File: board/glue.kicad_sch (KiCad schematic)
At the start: 25 parts, among them J1 Conn_01x05_Pin, J8 SD_Card_Receptacle, U12 GLUE, U13 SN74LVC245APW, U14 LD1117V33

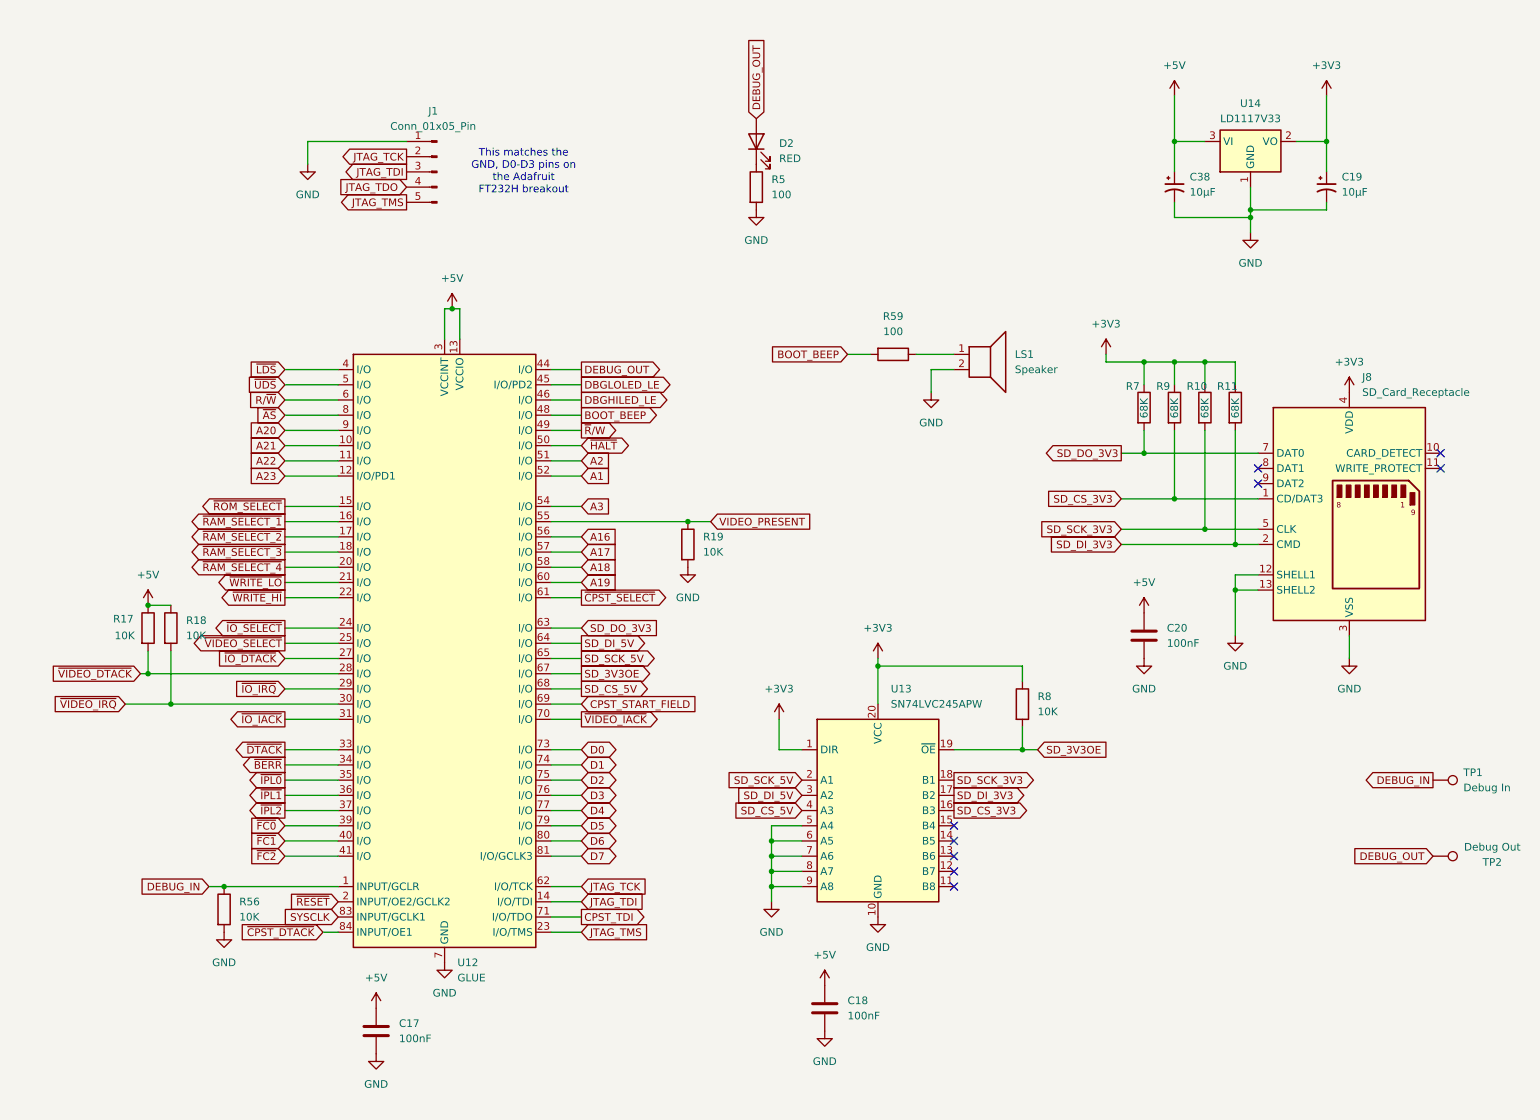
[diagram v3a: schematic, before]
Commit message: checkpoint before reordering 1508 inputs
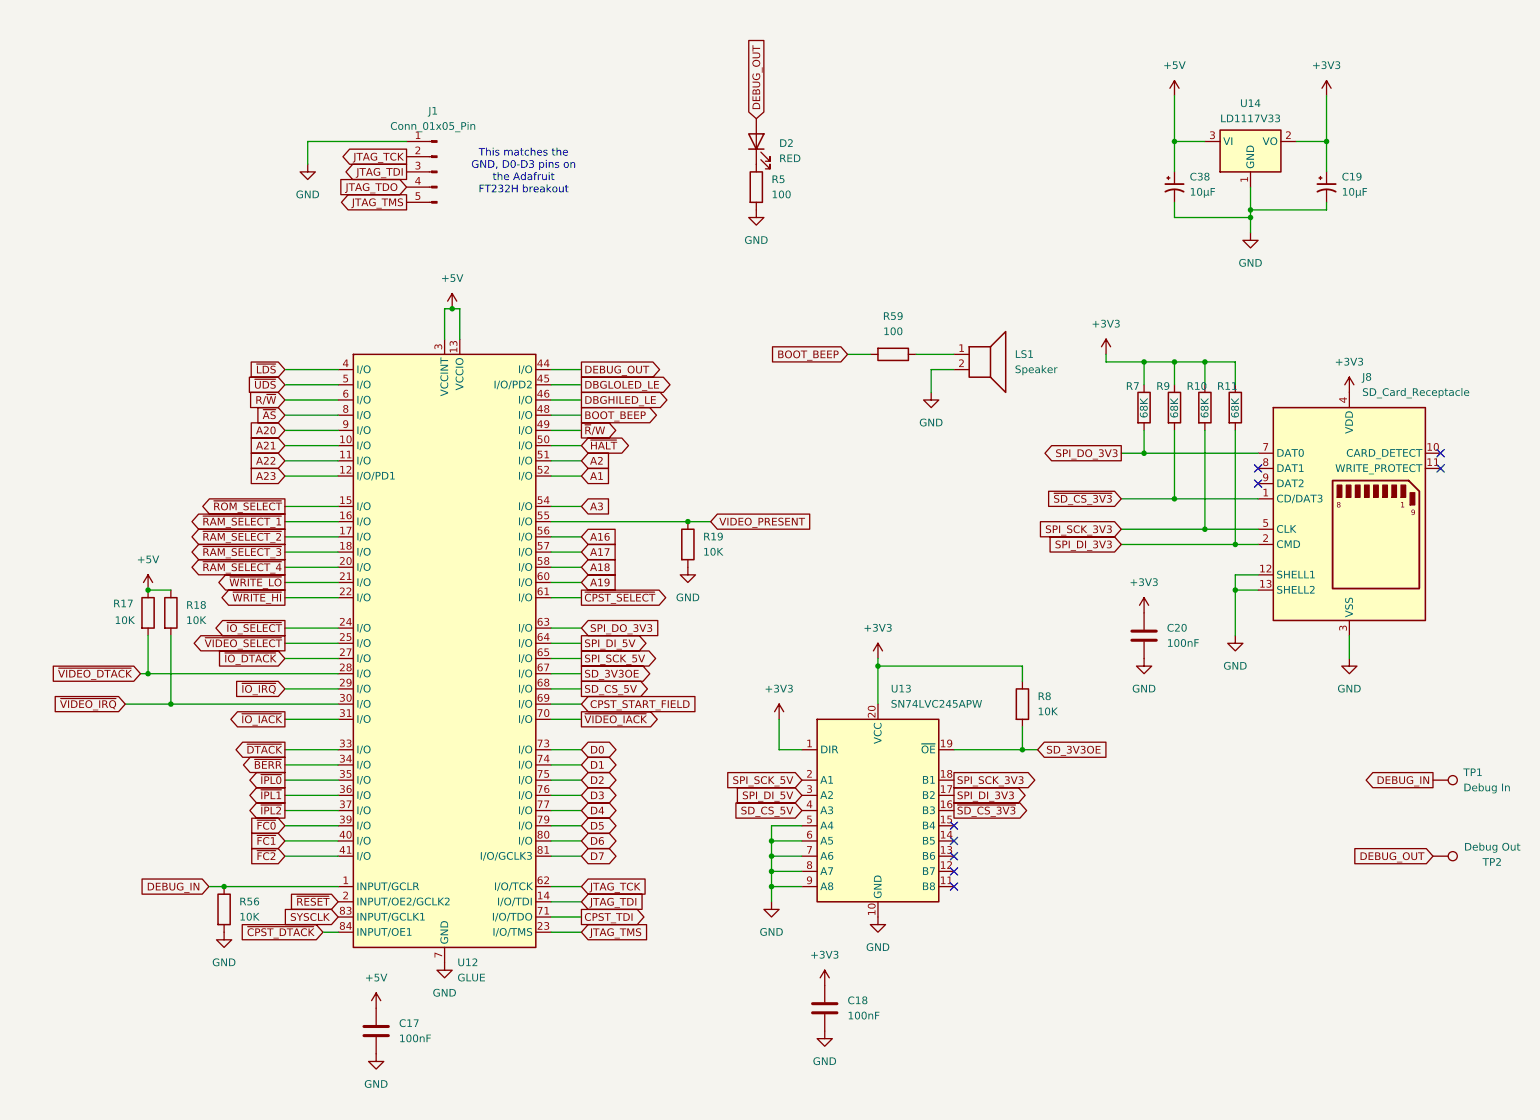
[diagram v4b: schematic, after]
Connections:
- net +3V3: now also C18.1, C20.1
- net +5V: no longer C18.1, C20.1
- net SD_CS_3V3 renamed ~{SD_CS_3V3}
- net SD_DI_3V3 renamed SPI_DI_3V3
- net SD_DI_5V renamed SPI_DI_5V
- net SD_DO_3V3 renamed SPI_DO_3V3
- net SD_SCK_3V3 renamed SPI_SCK_3V3
- net SD_SCK_5V renamed SPI_SCK_5V
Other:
- moved on the sheet: R17, R18
